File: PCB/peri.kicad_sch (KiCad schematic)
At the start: 3 parts, among them J1 Micro_SD_Card, U4 RN42

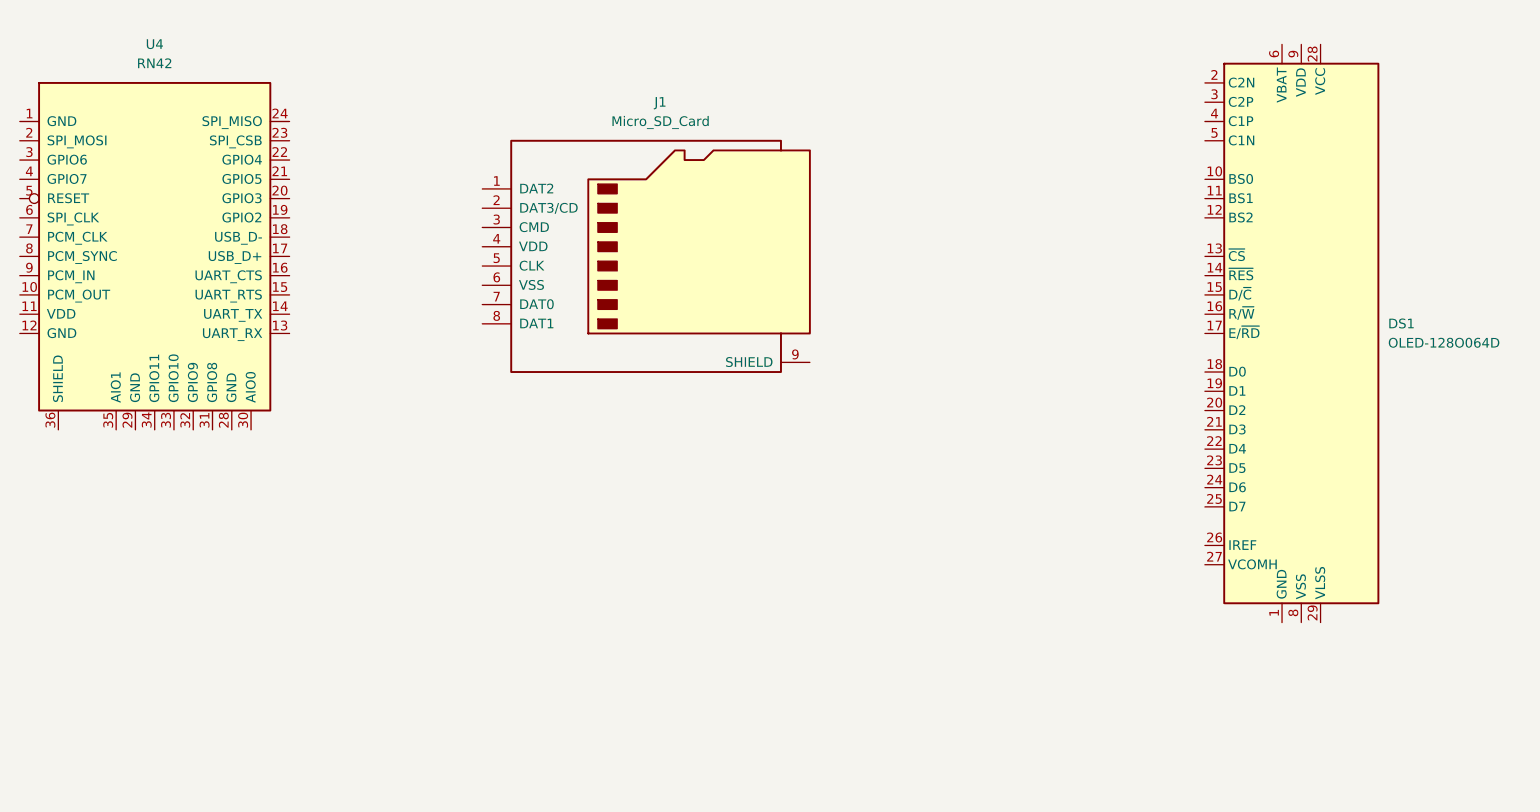
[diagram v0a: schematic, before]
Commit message: PCB init - Minh
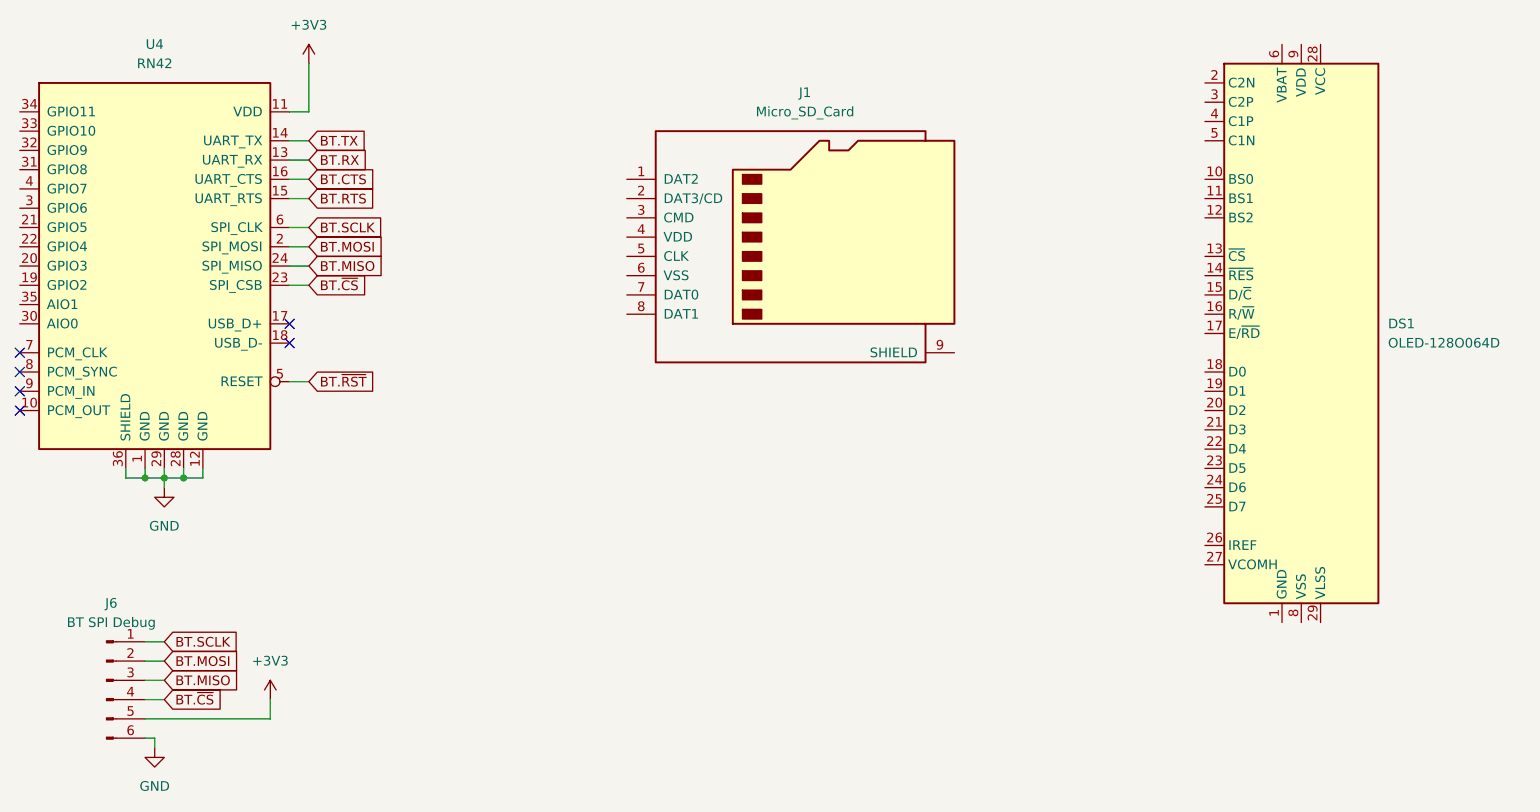
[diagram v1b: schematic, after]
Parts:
- added J6: BT SPI Debug, symbol Connector:Conn_01x06_Pin
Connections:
- net GND: now reaches U4.1 (GND)
- net GND: now also U4.12 (GND), U4.28 (GND), U4.29 (GND), U4.36 (SHIELD), J6.6 (Pin_6)
- net +3V3: now reaches U4.11 (VDD)
- net +3V3: now also J6.5 (Pin_5)
- net BT.RX: now reaches U4.13 (UART_RX)
- net BT.TX: now reaches U4.14 (UART_TX)
- net BT.RTS: now reaches U4.15 (UART_RTS)
- net BT.CTS: now reaches U4.16 (UART_CTS)
- net BT.MOSI: now reaches U4.2 (SPI_MOSI)
- net BT.MOSI: now also J6.2 (Pin_2)
- net BT.~{CS}: now reaches U4.23 (SPI_CSB)
- net BT.~{CS}: now also J6.4 (Pin_4)
- net BT.MISO: now reaches U4.24 (SPI_MISO)
- net BT.MISO: now also J6.3 (Pin_3)
- net BT.~{RST}: now reaches U4.5 (RESET)
- net BT.SCLK: now reaches U4.6 (SPI_CLK)
- net BT.SCLK: now also J6.1 (Pin_1)
- no-connect marks 0 -> 6
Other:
- moved on the sheet: J1, U4
